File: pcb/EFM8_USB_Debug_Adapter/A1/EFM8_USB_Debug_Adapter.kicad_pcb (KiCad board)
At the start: 2 copper layers, 55 x 45 mm, 36 parts, among them J100 EFM8_IDC_Debug_Header_Horizon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, J110 2137160001, J111 TTL-232R_Header_Horizontal, J120 31230102, J130 EFM8_USB_8-Bit_Debug_Header_H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, J131 Header_01x02_Wurth_61300211121, M110 USB_Light_Pipe, M120 PSU_Light_Pipe, M130 DBG8_Light_Pipe, Q110 SI3443CDV-T1-GE3, Q111 DMMT5401, Q120 SI3443CDV-T1-GE3, Q121 DMMT5401, Q130 SI3443CDV-T1-GE3, Q131 DMMT5401

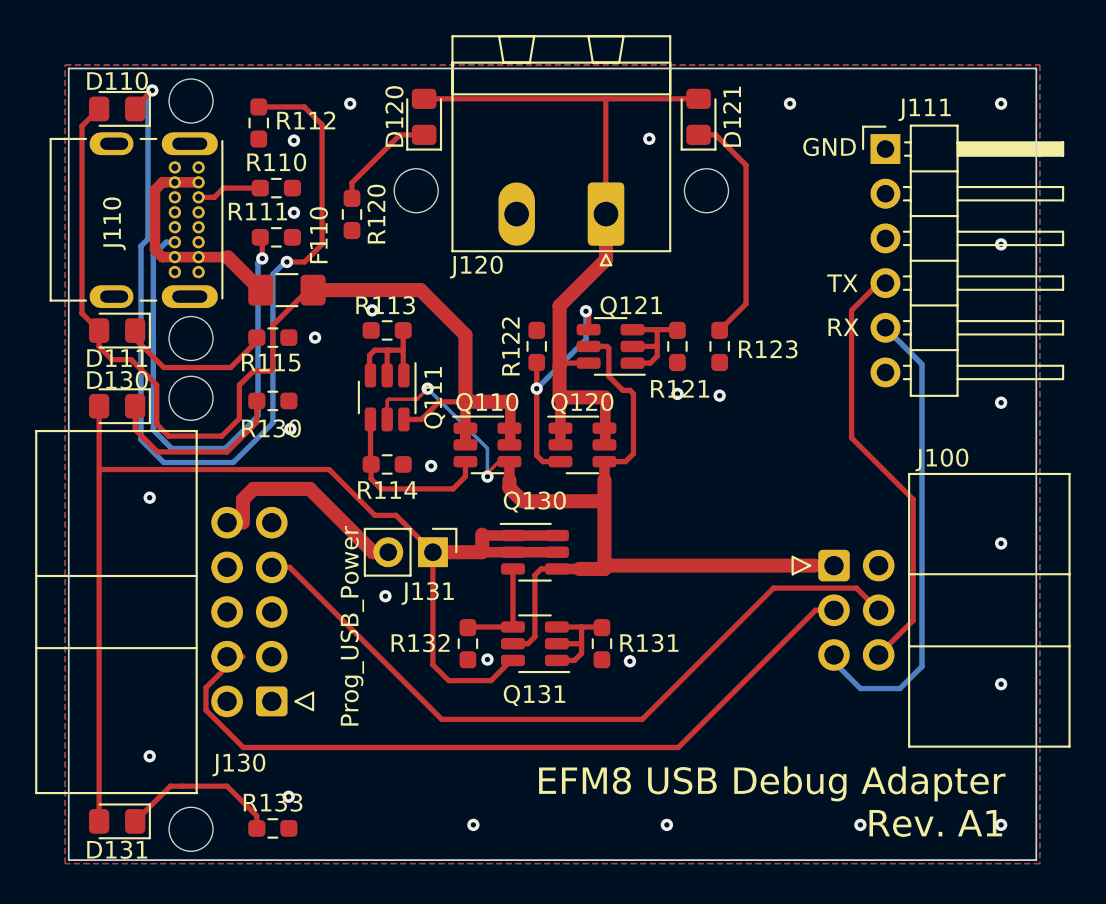
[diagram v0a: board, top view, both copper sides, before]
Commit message: PCB Rev. A1
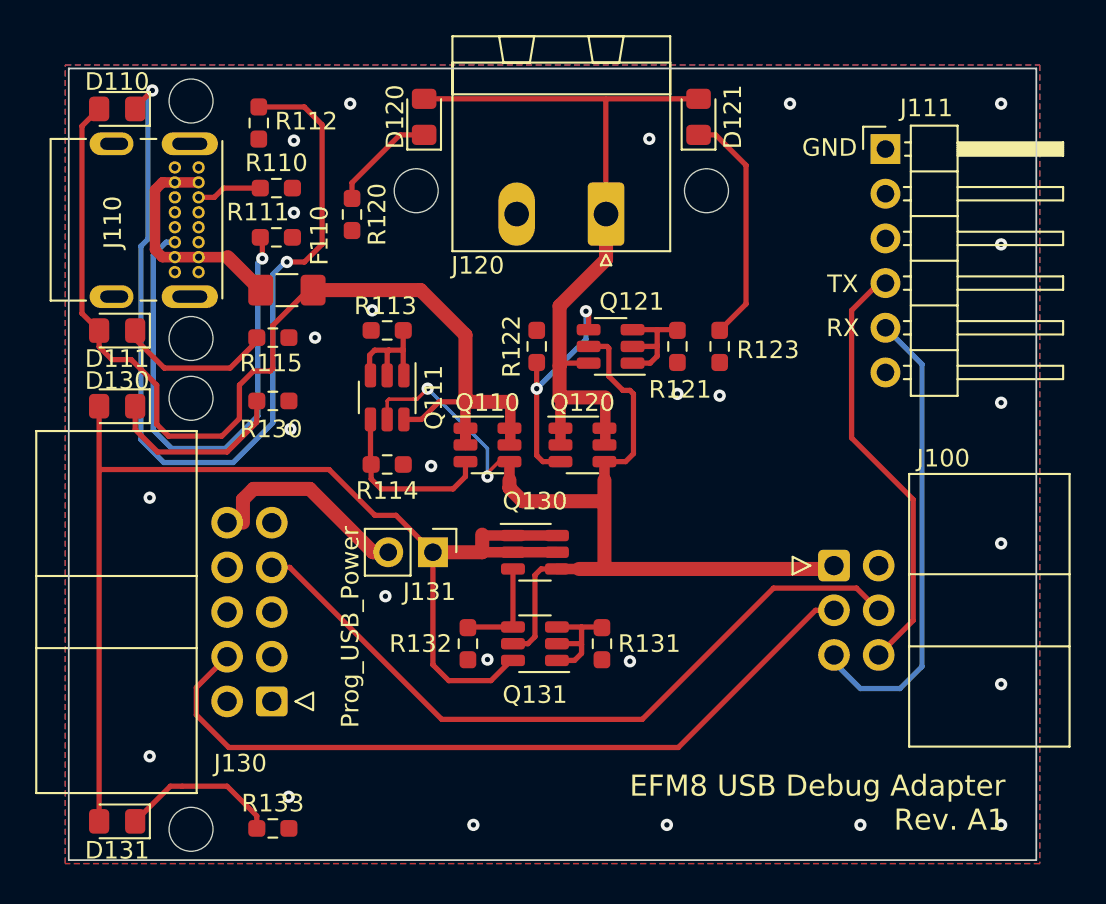
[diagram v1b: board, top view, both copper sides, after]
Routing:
- net /V_PROG: track 55.9 -> 57.0 mm
